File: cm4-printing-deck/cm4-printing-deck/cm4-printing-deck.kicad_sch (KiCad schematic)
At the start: 92 parts, among them J1 Micro_SD_Card, J10 KB_USB, J11 3-2328724-1, J12 MOLEX_503480-0600, J2 USB_C_Receptacle_USB2.0_14P, J3 PWR_BAT, J6 HDMI_A, J7 USB3_A, J8 USB3_A, SW20 Power, SW62 WIFIBT_DISABLE, U1 Compute_Module_4_Connectors, U10 CH32X05, U11 AP2112K-3.3, U12 SN74LVC1G34DBVRG4, U13 MCP23008T-E_SS, U14 AP1117-18, U2 AP64501SP-13, U3 RT9742GGJ5, U4 TPS784105QWDRBRQ1, U5 PCF85063ATL, U6 74LVC1G07, U7 74LVC1G07, U8 74LVC1G07, U9 VL805, Y2 Crystal_GND23, Y3 Crystal

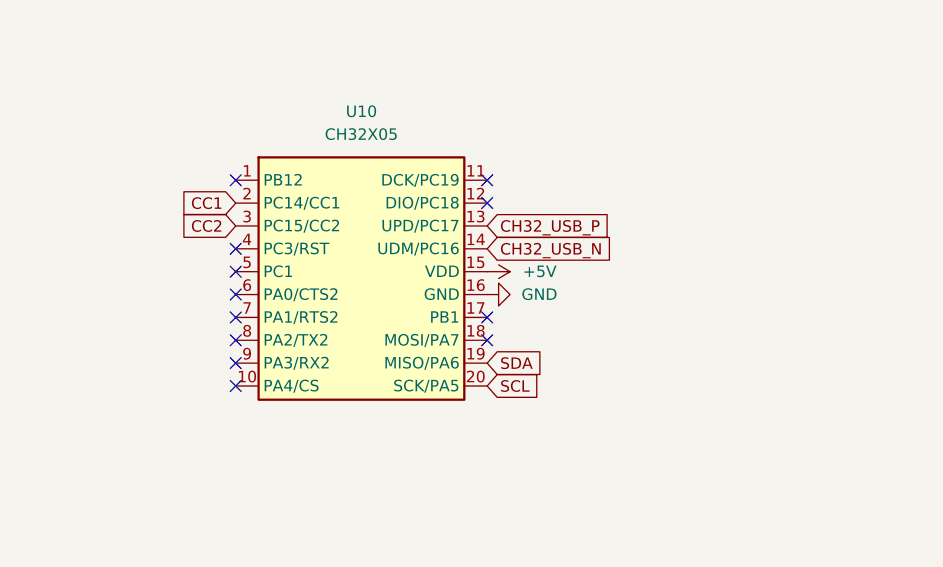
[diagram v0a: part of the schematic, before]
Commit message: add updated files
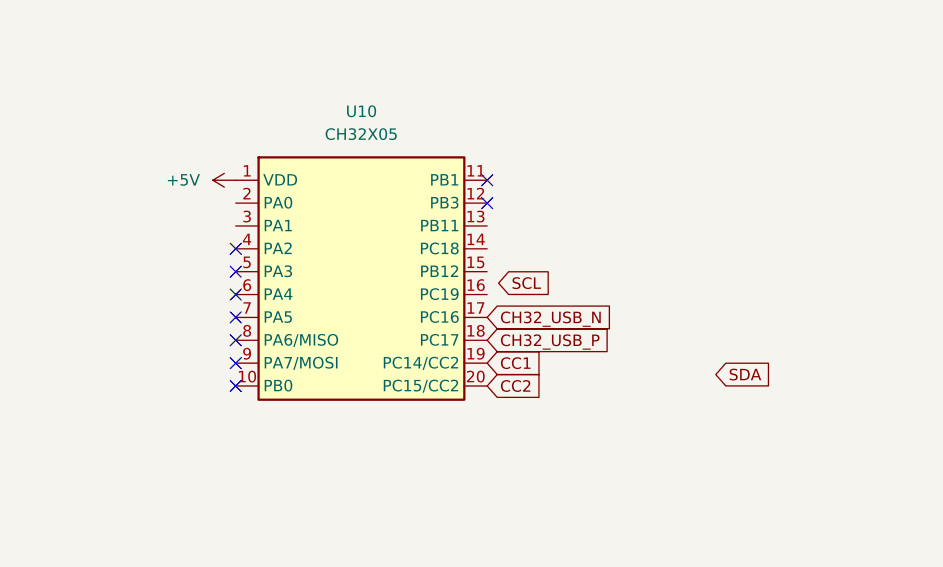
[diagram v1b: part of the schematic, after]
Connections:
- net +5V: now also U10.1 (VDD); no longer U10.15 (VDD)
- net CC1: now also U10.19 (PC14/CC2); no longer U10.2 (PC14/CC1)
- net CC2: now also U10.20 (PC15/CC2); no longer U10.3 (PC15/CC2)
- net CH32_USB_N: now also U10.17 (PC16); no longer U10.14 (UDM/PC16)
- net CH32_USB_P: now also U10.18 (PC17); no longer U10.13 (UPD/PC17)
- net GND: no longer U10.16 (GND)
- net SCL: no longer U10.20 (SCK/PA5)
- net SDA: no longer U10.19 (MISO/PA6)
- no-connect marks 142 -> 139
